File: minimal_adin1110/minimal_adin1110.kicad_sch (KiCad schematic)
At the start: 70 parts, among them J1 CLP-112-02-G-D-BE, J2 CLP-102-02-G-D-BE, J3 CLP-102-02-G-D-BE, J4 CLP-102-02-G-D-BE, J5 CLP-102-02-G-D-BE, U1 ADIN1110CCPZ, Y1 FA-128 25.0000MF20X-K0

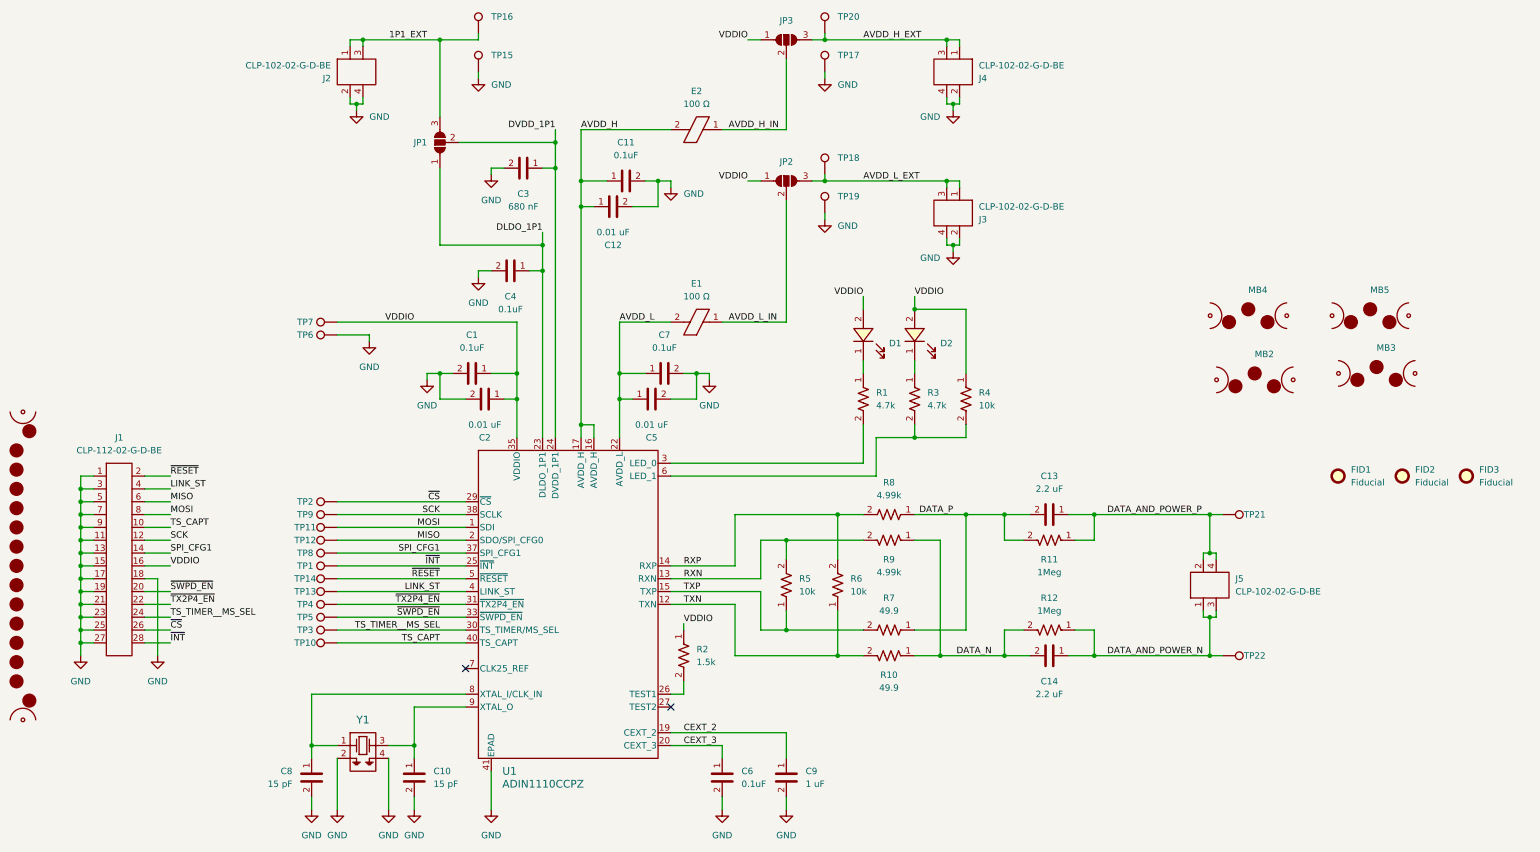
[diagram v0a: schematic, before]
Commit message: Update subproject commit for KiCAD Symbol Generator
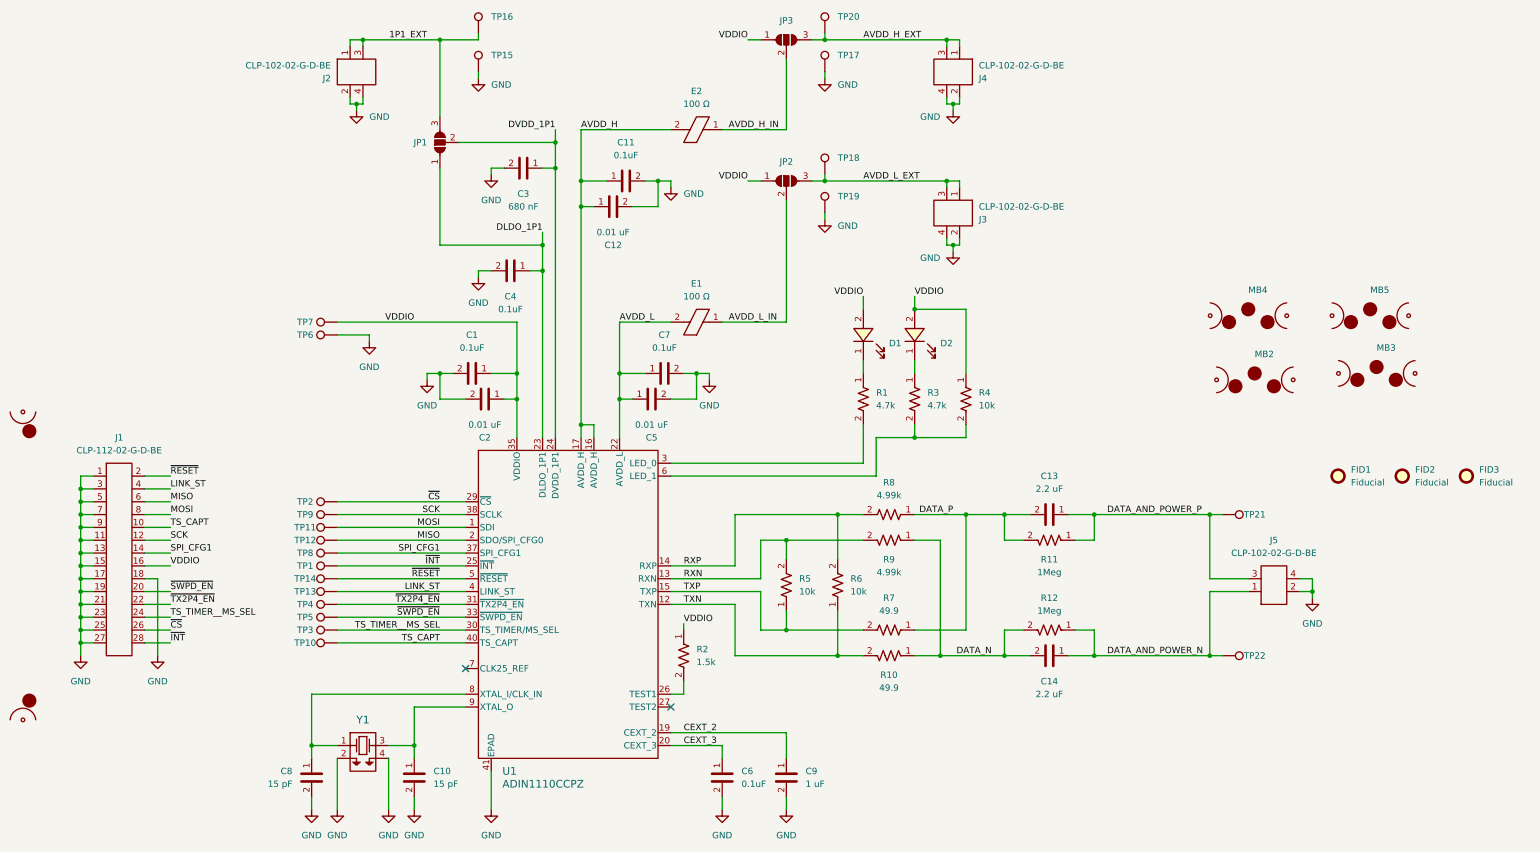
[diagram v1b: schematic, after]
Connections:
- net DATA_AND_POWER_N: no longer J5.3
- net DATA_AND_POWER_P: now also J5.3; no longer J5.2, J5.4
- net GND: now also J5.2, J5.4
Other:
- moved on the sheet: J5
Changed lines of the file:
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@@
 	)
 	(junction
-		(at 330.2 142.24)
-		(diameter 0)
-		(color 0 0 0 0)
-	)
-	(junction
 		(at 198.12 86.36)
 		(diameter 0)
@@
 	)
 	(junction
+		(at 350.52 149.86)
+		(diameter 0)
+		(color 0 0 0 0)
+	)
+	(junction
 		(at 278.13 40.64)
 		(diameter 0)
@@
 	)
 	(junction
-		(at 330.2 154.94)
-		(diameter 0)
-		(color 0 0 0 0)
-	)
-	(junction
 		(at 172.72 180.34)
 		(diameter 0)
@@
 	(wire
 		(pts
-			(xy 330.2 142.24) (xy 328.93 142.24)
+			(xy 109.22 142.24) (xy 106.68 142.24)
 		)
 		(stroke
@@
 	(wire
 		(pts
-			(xy 109.22 142.24) (xy 106.68 142.24)
+			(xy 303.53 157.48) (xy 307.34 157.48)
 		)
 		(stroke
@@
 	(wire
 		(pts
-			(xy 303.53 157.48) (xy 307.34 157.48)
+			(xy 109.22 149.86) (xy 106.68 149.86)
 		)
 		(stroke
@@
 	(wire
 		(pts
-			(xy 109.22 149.86) (xy 106.68 149.86)
+			(xy 254 48.26) (xy 254 46.99)
 		)
 		(stroke
@@
 	(wire
 		(pts
-			(xy 254 48.26) (xy 254 46.99)
+			(xy 106.68 132.08) (xy 106.68 134.62)
 		)
 		(stroke
@@
 	(wire
 		(pts
-			(xy 106.68 132.08) (xy 106.68 134.62)
+			(xy 177.8 66.04) (xy 177.8 81.28)
 		)
 		(stroke
@@
 	(wire
 		(pts
-			(xy 177.8 66.04) (xy 177.8 81.28)
+			(xy 347.98 149.86) (xy 350.52 149.86)
 		)
 		(stroke
@@
 	(wire
 		(pts
+			(xy 330.2 147.32) (xy 337.82 147.32)
+		)
+		(stroke
+			(width 0)
+			(type default)
+		)
+	)
+	(wire
+		(pts
 			(xy 223.52 111.76) (xy 228.6 111.76)
 		)
@@
 	(wire
 		(pts
+			(xy 347.98 147.32) (xy 350.52 147.32)
+		)
+		(stroke
+			(width 0)
+			(type default)
+		)
+	)
+	(wire
+		(pts
 			(xy 152.4 170.18) (xy 152.4 180.34)
 		)
@@
 	(wire
 		(pts
-			(xy 331.47 154.94) (xy 331.47 153.67)
+			(xy 330.2 149.86) (xy 330.2 162.56)
 		)
 		(stroke
@@
 	(wire
 		(pts
-			(xy 330.2 134.62) (xy 330.2 142.24)
+			(xy 350.52 151.13) (xy 350.52 149.86)
 		)
 		(stroke
@@
 	(wire
 		(pts
-			(xy 330.2 154.94) (xy 331.47 154.94)
-		)
-		(stroke
-			(width 0)
-			(type default)
-		)
-	)
-	(wire
-		(pts
 			(xy 271.78 91.44) (xy 271.78 93.98)
 		)
@@
 	(wire
 		(pts
-			(xy 330.2 154.94) (xy 330.2 162.56)
-		)
-		(stroke
-			(width 0)
-			(type default)
-		)
-	)
-	(wire
-		(pts
 			(xy 152.4 190.5) (xy 152.4 193.04)
 		)
@@
 	(wire
 		(pts
-			(xy 330.2 142.24) (xy 331.47 142.24)
-		)
-		(stroke
-			(width 0)
-			(type default)
-		)
-	)
-	(wire
-		(pts
 			(xy 254 76.2) (xy 254 74.93)
 		)
@@
 	(wire
 		(pts
-			(xy 328.93 143.51) (xy 328.93 142.24)
-		)
-		(stroke
-			(width 0)
-			(type default)
-		)
-	)
-	(wire
-		(pts
 			(xy 280.67 69.85) (xy 280.67 68.58)
 		)
@@
 	(wire
 		(pts
-			(xy 331.47 142.24) (xy 331.47 143.51)
+			(xy 330.2 134.62) (xy 330.2 147.32)
 		)
 		(stroke
@@
 	(wire
 		(pts
-			(xy 328.93 154.94) (xy 330.2 154.94)
-		)
-		(stroke
-			(width 0)
-			(type default)
-		)
-	)
-	(wire
-		(pts
 			(xy 198.12 81.28) (xy 198.12 86.36)
 		)
@@
 	(wire
 		(pts
-			(xy 328.93 153.67) (xy 328.93 154.94)
-		)
-		(stroke
-			(width 0)
-			(type default)
-		)
-	)
-	(wire
-		(pts
 			(xy 271.78 134.62) (xy 281.94 134.62)
 		)
@@
 	(wire
 		(pts
+			(xy 330.2 149.86) (xy 337.82 149.86)
+		)
+		(stroke
+			(width 0)
+			(type default)
+		)
+	)
+	(wire
+		(pts
 			(xy 226.06 106.68) (xy 228.6 106.68)
 		)
@@
 	(wire
 		(pts
+			(xy 350.52 147.32) (xy 350.52 149.86)
+		)
+		(stroke
+			(width 0)
+			(type default)
+		)
+	)
+	(wire
+		(pts
 			(xy 220.98 68.58) (xy 220.98 73.66)
 		)
@@
 	(symbol
 		(lib_id "UNITED_CONNECTORS_DATA_BASE:J_CLP-102-02-G-D-BE")
-		(at 330.2 148.59 90)
+		(at 342.9 148.59 0)
+		(mirror x)
 		(unit 1)
 		(exclude_from_sim no)
@@
 		(on_board yes)
 		(dnp no)
-		(fields_autoplaced yes)
 		(property "Reference" "J5"
-			(at 335.28 147.3199 90)
+			(at 342.9 139.7 0)
 			(effects
 				(font
 					(size 1.27 1.27)
 				)
-				(justify right)
 			)
 		)
 		(property "Value" "CLP-102-02-G-D-BE"
-			(at 335.28 149.8599 90)
+			(at 342.9 142.24 0)
 			(effects
 				(font
 					(size 1.27 1.27)
 				)
-				(justify right)
 			)
 		)
 		(property "Footprint" "connector_footprints:CLP-102-02-G-D-BE"
-			(at 337.82 143.51 0)
+			(at 347.98 140.97 0)
 			(show_name yes)
 			(effects
@@
 		)
 		(property "Datasheet" "https://suddendocs.samtec.com/catalog_english/clp_sm.pdf?_gl=1*1y4jlr9*_gcl_au*MTM0MTYyNTQ5MS4xNzM2MDk5MTUz*_ga*MTYxNDYyMTQ0Mi4xNzM2MDk5MTUz*_ga_3KFNZC07WW*MTczNjY4MDQ4OS4xNS4xLjE3MzY2ODEzNzcuNjAuMC4w"
-			(at 340.36 143.51 0)
+			(at 347.98 138.43 0)
 			(show_name yes)
 			(effects
@@
 		)
 		(property "Description" "Samtec CLP-1xx-02-G-D-BE series,  2 positions connector,  1.27 mm pitch,  Black,  Vertical mounting,  5.2 A,  300 V,  Through Hole,  Tin plated"
-			(at 342.9 143.51 0)
+			(at 347.98 135.89 0)
 			(show_name yes)
 			(effects
@@
 		)
 		(property "Color" "Black"
-			(at 345.44 143.51 0)
+			(at 347.98 133.35 0)
 			(show_name yes)
 			(effects
@@
 		)
 		(property "Contact Plating" "Tin"
-			(at 347.98 143.51 0)
+			(at 347.98 130.81 0)
 			(show_name yes)
 			(effects
@@
 		)
 		(property "Current Rating (A)" "5.2"
-			(at 350.52 143.51 0)
+			(at 347.98 128.27 0)
 			(show_name yes)
 			(effects
@@
 		)
 		(property "MPN" "CLP-102-02-G-D-BE"
-			(at 353.06 143.51 0)
+			(at 347.98 125.73 0)
 			(show_name yes)
 			(effects
@@
 		)
 		(property "Manufacturer" "Samtec"
-			(at 355.6 143.51 0)
+			(at 347.98 123.19 0)
 			(show_name yes)
 			(effects
@@
 		)
 		(property "Mounting Angle" "Vertical"
-			(at 358.14 143.51 0)
+			(at 347.98 120.65 0)
 			(show_name yes)
 			(effects
@@
 		)
 		(property "Mounting Style" "Through Hole"
-			(at 360.68 143.51 0)
+			(at 347.98 118.11 0)
 			(show_name yes)
 			(effects
@@
 		)
 		(property "Number of Rows" "2"
-			(at 363.22 143.51 0)
+			(at 347.98 115.57 0)
 			(show_name yes)
 			(effects
@@
 		)
 		(property "Pin Count" "2"
-			(at 365.76 143.51 0)
+			(at 347.98 113.03 0)
 			(show_name yes)
 			(effects
@@
 		)
 		(property "Pitch (mm)" "1.27"
-			(at 368.3 143.51 0)
+			(at 347.98 110.49 0)
 			(show_name yes)
 			(effects
@@
 		)
 		(property "Series" "CLP-1xx-02-G-D-BE"
-			(at 370.84 143.51 0)
+			(at 347.98 107.95 0)
 			(show_name yes)
 			(effects
@@
 		)
 		(property "Symbol Name" "J_CLP-102-02-G-D-BE"
-			(at 373.38 143.51 0)
+			(at 347.98 105.41 0)
 			(show_name yes)
 			(effects
@@
 		)
 		(property "Trustedparts Search" "https://www.trustedparts.com/en/search/CLP-102-02-G-D-BE"
-			(at 375.92 143.51 0)
+			(at 347.98 102.87 0)
 			(show_name yes)
 			(effects
@@
 		)
 		(property "Voltage Rating (V)" "300"
-			(at 378.46 143.51 0)
+			(at 347.98 100.33 0)
 			(show_name yes)
 			(effects
@@
 					(unit 1)
 				)
+			)
+		)
+	)
+	(symbol
+		(lib_id "power:GND")
+		(at 350.52 151.13 0)
+		(unit 1)
+		(exclude_from_sim no)
+		(in_bom yes)
+		(on_board yes)
+		(dnp no)
+		(fields_autoplaced yes)
+		(property "Reference" "#PWR22"
+			(at 350.52 157.48 0)
+			(effects
+				(font
+					(size 1.27 1.27)
+				)
+				(hide yes)
+			)
+		)
+		(property "Value" "GND"
+			(at 350.52 156.21 0)
+			(effects
+				(font
+					(size 1.27 1.27)
+				)
+			)
+		)
+		(property "Footprint" ""
+			(at 350.52 151.13 0)
+			(effects
+				(font
+					(size 1.27 1.27)
+				)
+				(hide yes)
+			)
+		)
+		(property "Datasheet" ""
+			(at 350.52 151.13 0)
+			(effects
+				(font
+					(size 1.27 1.27)
+				)
+				(hide yes)
+			)
+		)
+		(property "Description" "Power symbol creates a global label with name \"GND\" , ground"
+			(at 350.52 151.13 0)
+			(effects
+				(font
+					(size 1.27 1.27)
+				)
+				(hide yes)
+			)
+		)
+		(pin "1"
+		)
+		(instances
+			(project "minimal_adin1110"
+				(path "/26ddf1b8-aee4-468d-a26c-7bd63f3a2989"
+					(reference "#PWR22")
+					(unit 1)
+				)
